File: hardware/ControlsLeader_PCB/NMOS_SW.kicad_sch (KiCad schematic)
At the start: 4 parts, among them Q15 NMOS

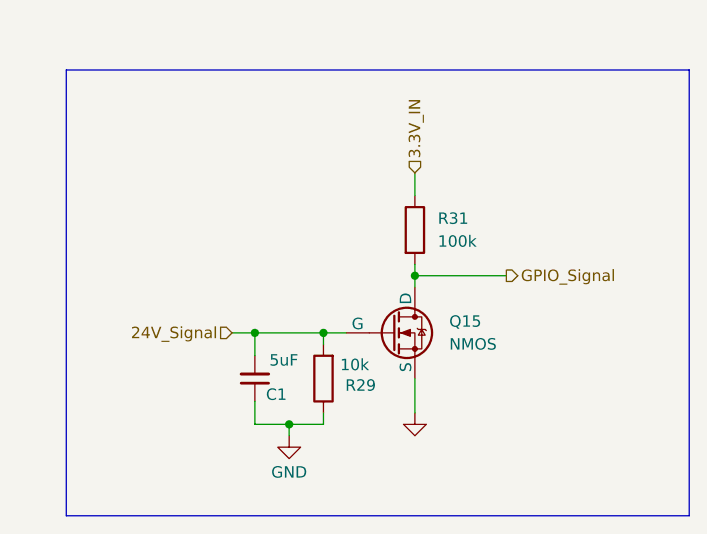
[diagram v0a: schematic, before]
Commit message: DONE!!! - just need to add footprints + part #s)
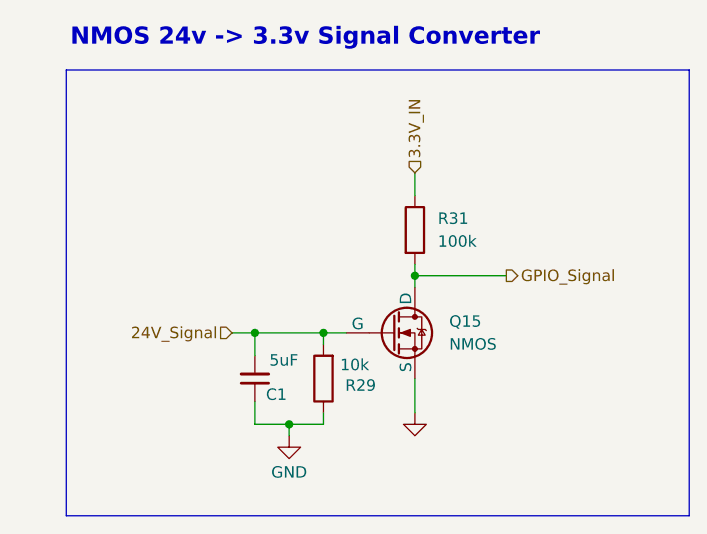
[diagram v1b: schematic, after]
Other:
- note added: "NMOS 24v -> 3.3v Signal Converter"
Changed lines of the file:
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@@
+		)
+	)
+	(text "NMOS 24v -> 3.3v Signal Converter"
+		(exclude_from_sim no)
+		(at 141.478 70.104 0)
+		(effects
+			(font
+				(size 1.905 1.905)
+				(thickness 0.254)
+				(bold yes)
+			)
 		)
 	)
